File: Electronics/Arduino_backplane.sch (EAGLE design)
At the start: 36 parts, among them IC1 4013N, IC2 MCP4802, IC3 MCP4802, Q1 BF199, Q5 BF199, X1 M25-HD-20, X2 M25-HD-20

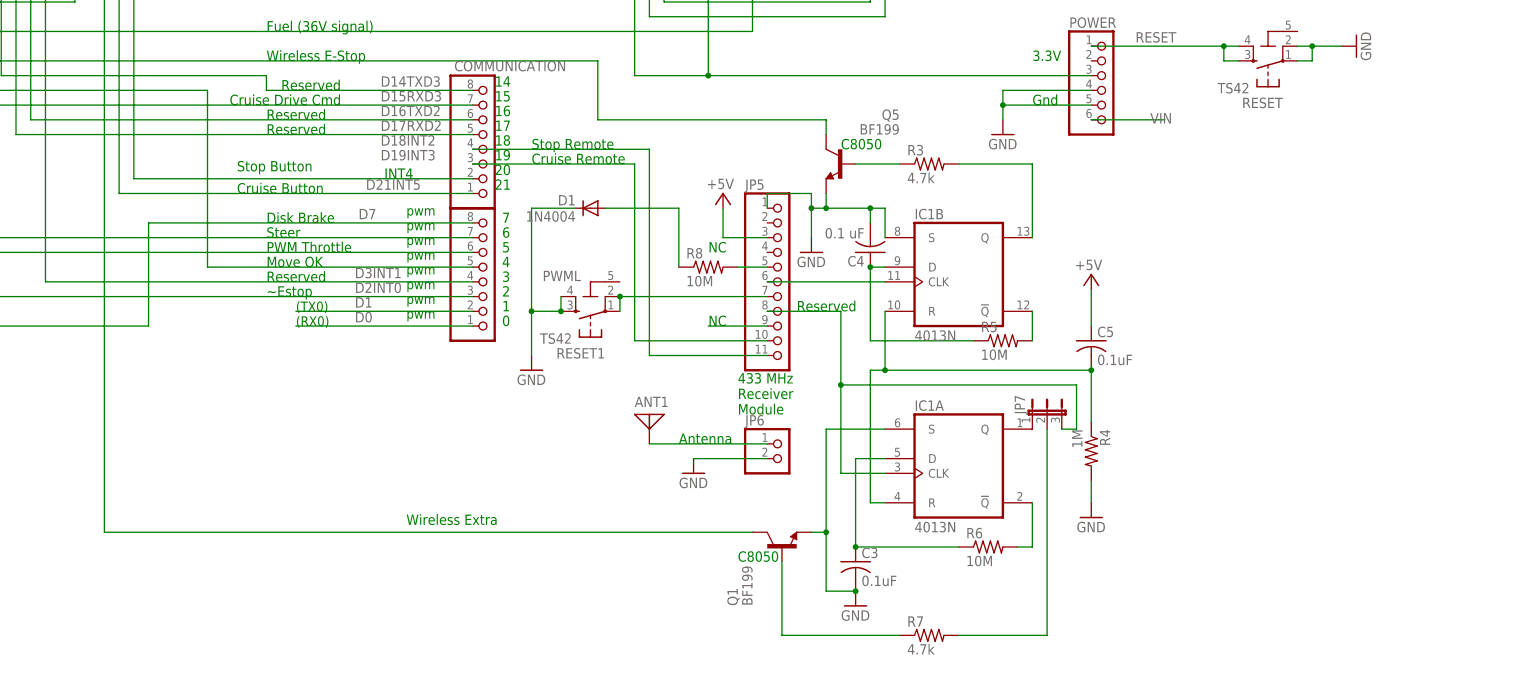
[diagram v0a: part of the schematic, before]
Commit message: Modifications by Tyler and Charles on March 14.
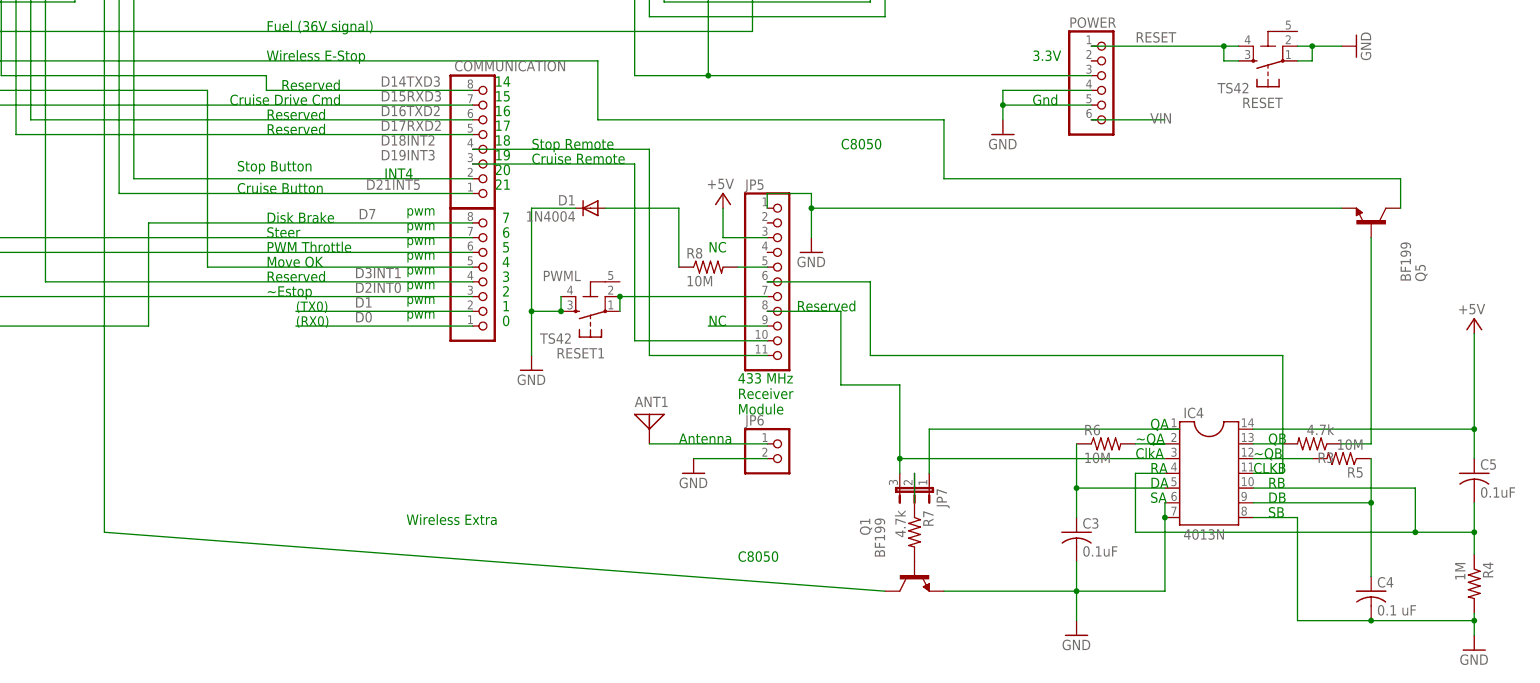
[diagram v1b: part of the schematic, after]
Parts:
- removed IC1: 4013N, 40xx:4013N
- added IC4: 4013N, ic-package:DIL14
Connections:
- removed net N$2: C4.1, IC1B.D, R5.1
- removed net N$25: IC1B.CLK, JP5.6
- removed net N$27: JP7.2, R7.2
- removed net N$30: IC1A.CLK, JP5.8, JP7.3
- removed net N$34: IC1B.!Q, R5.2
- removed net N$35: C3.1, IC1A.D, R6.1
- removed net N$36: C5.2, IC1A.R, IC1B.R, R4.1
- removed net N$38: IC1A.!Q, R6.2
- removed net N$39: Q1.B, R7.1
- removed net N$4: IC1A.Q, JP7.1
- removed net N$5: IC1B.Q, R3.2
- new net CLKA: IC4.3, JP5.8, JP7.3
- new net CLKB: IC4.11, JP5.6
- new net DA: C3.1, IC4.5, R6.1
- new net DB: C4.1, IC4.9, R5.1
- new net N$11: JP7.2, R7.1
- new net N$12: Q1.B, R7.2
- new net QA: IC4.1, JP7.1
- new net QB: R3.2
- new net RA: C5.2, IC4.10, IC4.4, R4.1
- new net ~QA: IC4.2, R6.2
- new net ~QB: IC4.12, R5.2
- net +5V: now also IC4.14
- net GND: now also IC4.6, IC4.7, IC4.8; no longer IC1A.S, IC1B.S
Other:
- note added: "CLKB"
- note added: "ClkA"
- note added: "DA"
- note added: "DB"
- note added: "QA"
- note added: "QB"
- note added: "RA"
- note added: "RB"
- note added: "SA"
- note added: "SB"
- note added: "~QA"
- note added: "~QB"
- moved on the sheet: C3, C4, C5, JP7, Q1, Q5, R3, R4, R5, R6, R7
